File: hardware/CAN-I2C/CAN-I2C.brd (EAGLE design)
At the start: 90.2 x 15.2 mm, 31 parts, among them Q1 12MHZ, U1 MCP2515(MCP2510)ML, U2 MCP2551, U4 ATTINY816M

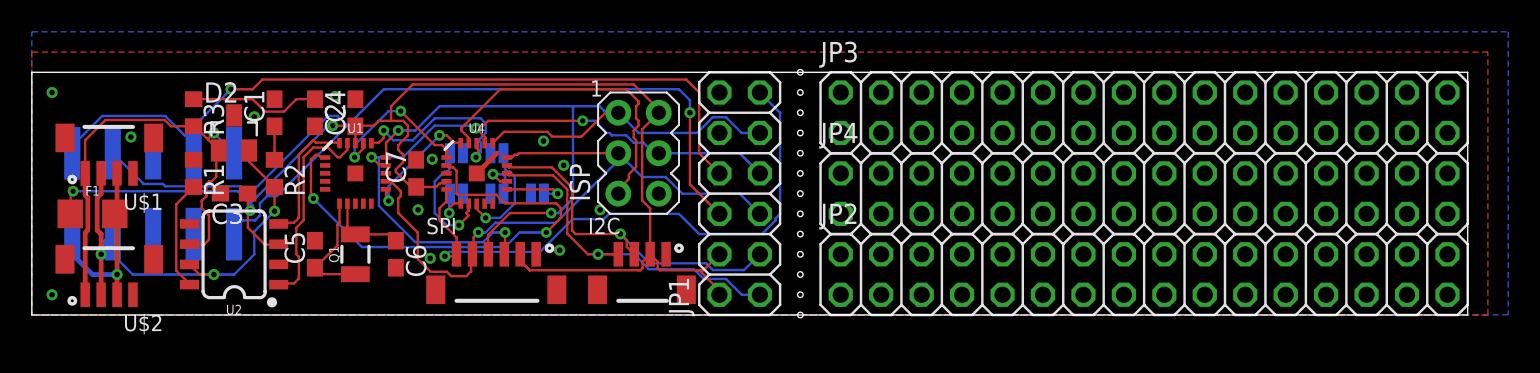
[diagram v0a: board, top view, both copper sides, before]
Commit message: Re-arranging directory structure
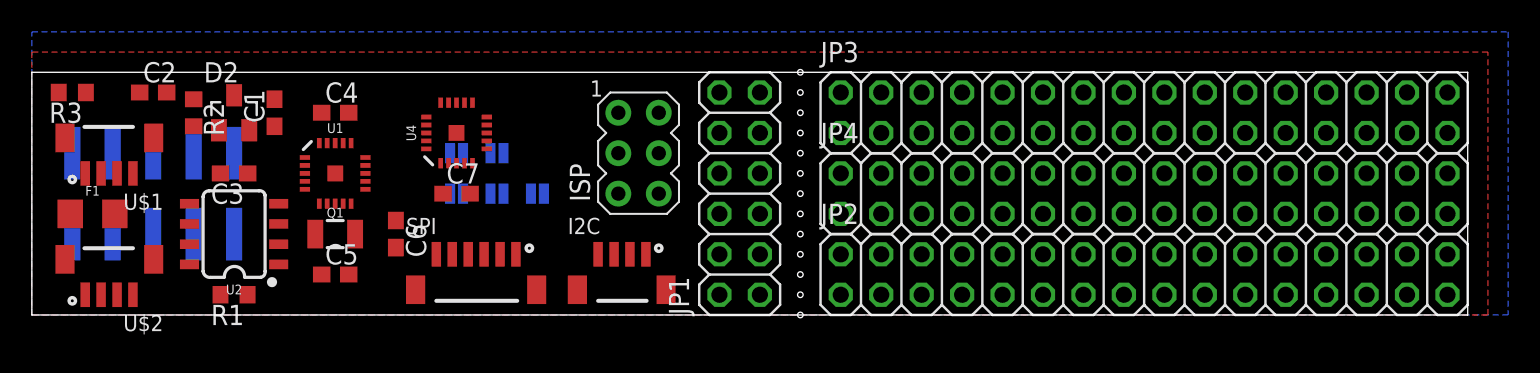
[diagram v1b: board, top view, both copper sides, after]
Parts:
- moved C2 10.2 mm to (7.62, 14.0), turned to 0 degrees
- moved R1 8.03 mm to (12.7, 1.27), turned to 180 degrees
- moved R3 7.73 mm to (2.54, 14.0), turned to 180 degrees
- moved R2 6.35 mm to (10.2, 12.7)
- moved C7 2.84 mm to (26.7, 7.62), turned to 0 degrees
- moved U4 2.84 mm to (26.7, 11.4), turned to 90 degrees
- moved C5 1.80 mm to (19.1, 2.54), turned to 0 degrees
- moved Q1 1.80 mm to (19.1, 5.08), turned to 0 degrees
- moved SPI 1.27 mm to (25.4, 3.81)
- moved C3 1.27 mm to (12.7, 8.89)
- moved C6 1.27 mm to (22.9, 5.08)
- moved U2 1.27 mm to (12.7, 5.08)
- moved C4 1.27 mm to (19.1, 12.7), turned to 0 degrees
- moved D2 1.27 mm to (12.7, 12.7)
- moved U1 1.27 mm to (19.1, 8.89)
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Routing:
- net +3V3: track 84.7 -> 0.00 mm, vias 3 -> 0
- net +5V: track 59.0 -> 0.00 mm, vias 1 -> 0
- net +12V: track 51.1 -> 0.00 mm, vias 1 -> 0
- net MISO: track 49.1 -> 0.00 mm, vias 2 -> 0
- net MOSI: track 42.9 -> 0.00 mm, vias 4 -> 0
- net SCK: track 41.5 -> 0.00 mm, vias 1 -> 0
- net !OUT_CS!: track 36.9 -> 0.00 mm, vias 1 -> 0
- net CLK: track 30.9 -> 0.00 mm, vias 2 -> 0
- net N$4: track 30.1 -> 0.00 mm, vias 3 -> 0
- net N$5: track 29.6 -> 0.00 mm, vias 1 -> 0
- net SCL: track 22.4 -> 0.00 mm, vias 1 -> 0
- net SDA: track 21.9 -> 0.00 mm, vias 1 -> 0
- net RST: track 20.2 -> 0.00 mm
- net N$2: track 13.2 -> 0.00 mm
- net N$13: track 12.4 -> 0.00 mm, vias 1 -> 0
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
